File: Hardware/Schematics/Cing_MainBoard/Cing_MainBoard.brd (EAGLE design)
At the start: 100 x 100 mm, 168 parts, among them IC1 L293D, IC2 LM2576S, IC3 FT232RL, IC5 BME280, Q1 16mhz, Q2 BSS138, Q3 BSS138, Q4 BSS138, Q5 BSS138, Q6 NP2301AMR-G, Q7 NP2301AMR-G, U3 MPU-6050MPU6050

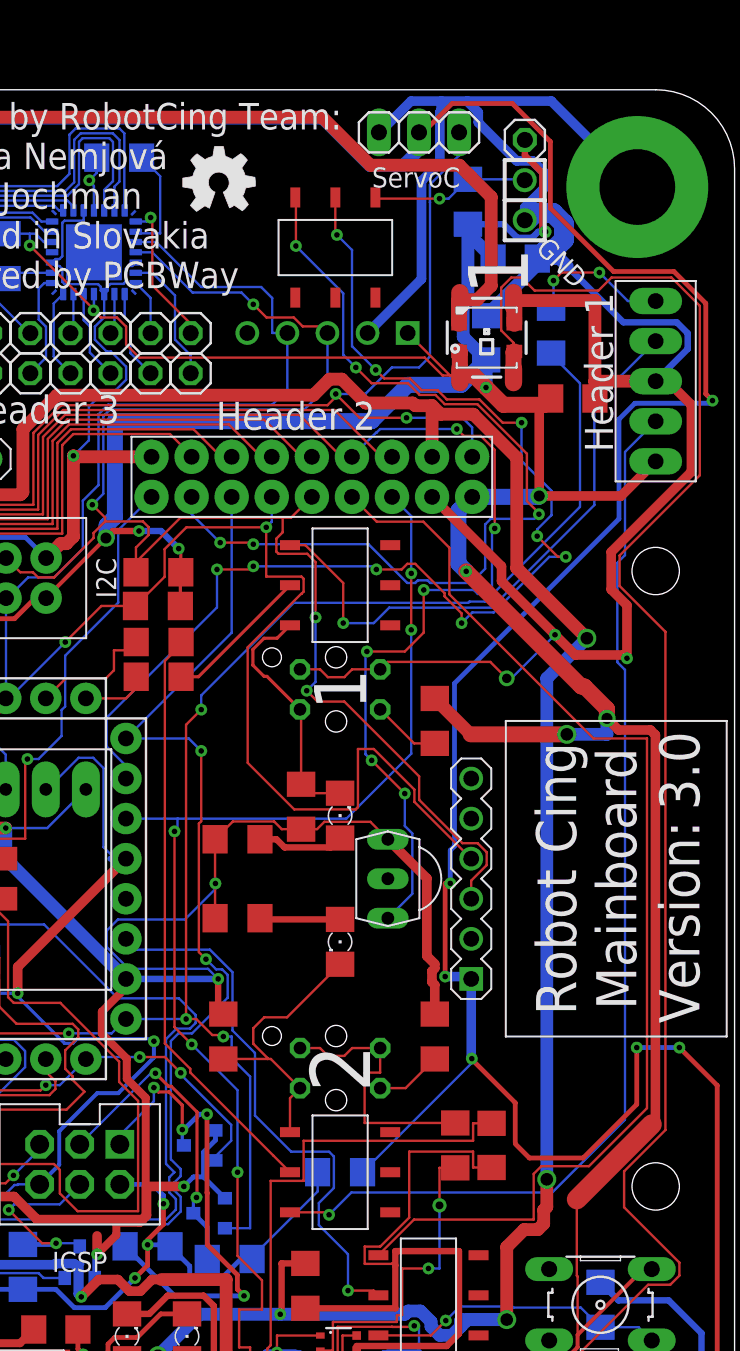
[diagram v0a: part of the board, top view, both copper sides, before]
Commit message: c
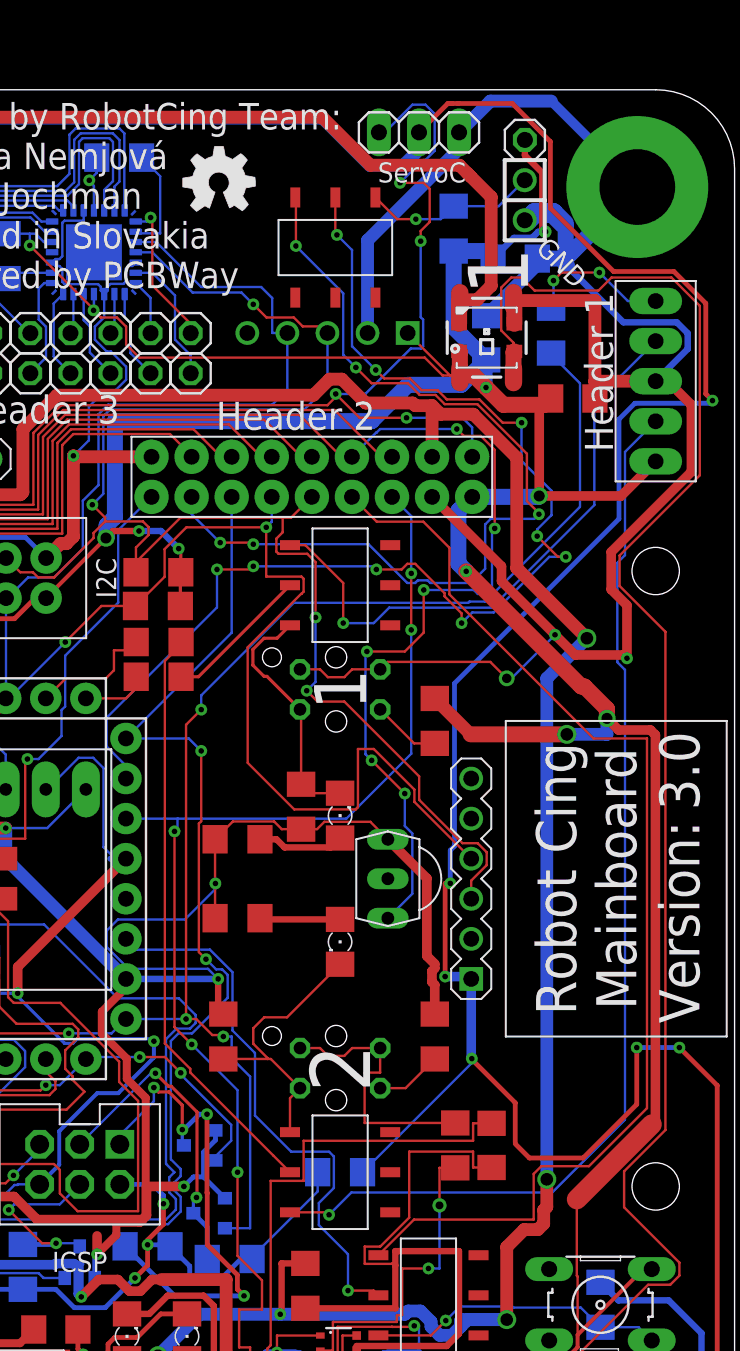
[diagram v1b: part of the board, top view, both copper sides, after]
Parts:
- moved R29 1.92 mm to (32.2, 41.2)
- turned JP4 to 0 degrees
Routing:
- net GND: track 865.0 -> 853.4 mm
- net D6: track 119.5 -> 126.5 mm, vias 3 -> 5
- net +3V3: track 671.7 -> 668.5 mm
- net N$66: track 10.0 -> 11.1 mm
